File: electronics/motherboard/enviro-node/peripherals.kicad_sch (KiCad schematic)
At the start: 9 parts, among them J5 ST1W008S4AR1500, J6 2604-3105, Q3 BSS214NW, U3 TCA9534

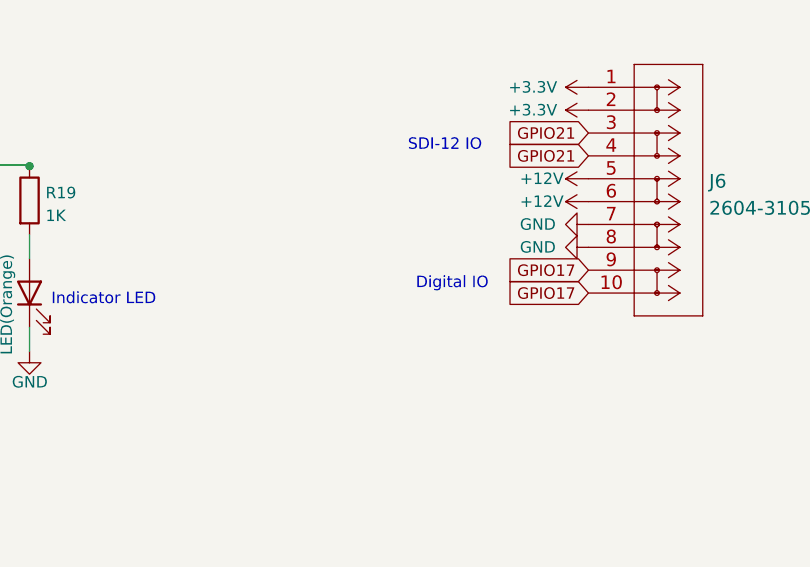
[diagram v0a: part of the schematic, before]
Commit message: updated electronics for production
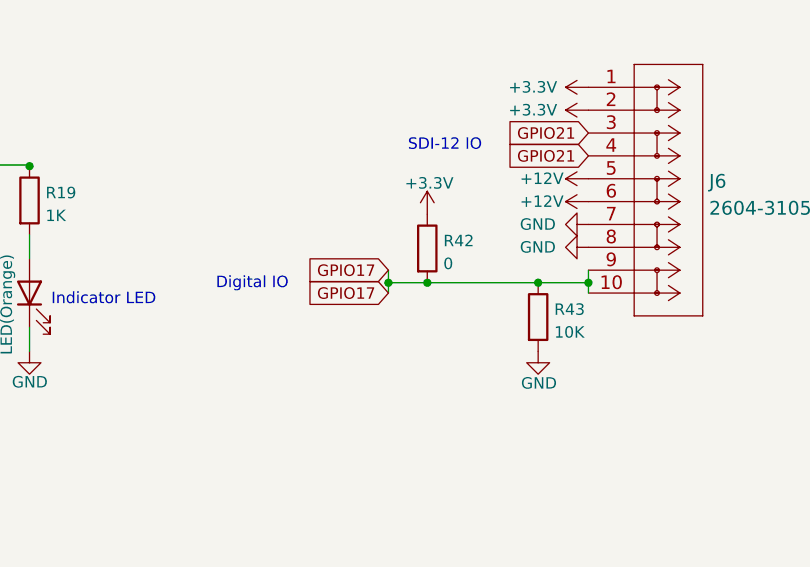
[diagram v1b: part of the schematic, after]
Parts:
- added R42: 0, Resistor_SMD:R_0805_2012Metric, symbol Device:R
- added R43: 10K, Resistor_SMD:R_0805_2012Metric, symbol Device:R
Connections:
- net +3.3V: now also R42.1
- net GND: now also R43.2
- net GPIO17: now also R42.2, R43.1
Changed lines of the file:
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@@
   (junction (at 119.507 115.697) (diameter 0) (color 0 0 0 0)
   )
+  (junction (at 230.632 116.078) (diameter 0) (color 0 0 0 0)
+  )
+  (junction (at 213.995 116.078) (diameter 0) (color 0 0 0 0)
+  )
   (junction (at 119.507 118.237) (diameter 0) (color 0 0 0 0)
   )
   (junction (at 174.117 103.124) (diameter 0) (color 0 0 0 0)
+  )
+  (junction (at 218.313 116.078) (diameter 0) (color 0 0 0 0)
+  )
+  (junction (at 236.22 116.078) (diameter 0) (color 0 0 0 0)
   )
   (no_connect (at 119.507 105.537))
@@
     (stroke (width 0) (type default) (color 0 0 0 0))
   )
+  (wire (pts (xy 236.22 114.681) (xy 236.22 116.078))
+    (stroke (width 0) (type default) (color 0 0 0 0))
+  )
+  (wire (pts (xy 213.995 116.078) (xy 213.995 117.221))
+    (stroke (width 0) (type default) (color 0 0 0 0))
+  )
   (wire (pts (xy 58.928 104.902) (xy 46.101 104.902))
     (stroke (width 0) (type default) (color 0 0 0 0))
   )
+  (wire (pts (xy 213.995 116.078) (xy 218.313 116.078))
+    (stroke (width 0) (type default) (color 0 0 0 0))
+  )
   (wire (pts (xy 174.117 102.997) (xy 174.117 103.124))
     (stroke (width 0) (type default) (color 0 0 0 0))
@@
     (stroke (width 0) (type default) (color 0 0 0 0))
   )
+  (wire (pts (xy 236.22 116.078) (xy 236.22 117.221))
+    (stroke (width 0) (type default) (color 0 0 0 0))
+  )
+  (wire (pts (xy 230.632 116.078) (xy 236.22 116.078))
+    (stroke (width 0) (type default) (color 0 0 0 0))
+  )
   (wire (pts (xy 58.928 125.222) (xy 58.928 104.902))
     (stroke (width 0) (type default) (color 0 0 0 0))
   )
+  (wire (pts (xy 218.313 116.078) (xy 230.632 116.078))
+    (stroke (width 0) (type default) (color 0 0 0 0))
+  )
   (wire (pts (xy 139.827 102.997) (xy 174.117 102.997))
     (stroke (width 0) (type default) (color 0 0 0 0))
   )
+  (wire (pts (xy 213.995 114.681) (xy 213.995 116.078))
+    (stroke (width 0) (type default) (color 0 0 0 0))
+  )
   (wire (pts (xy 119.507 115.697) (xy 119.507 118.237))
     (stroke (width 0) (type default) (color 0 0 0 0))
@@
     (stroke (width 0) (type default) (color 0 0 0 0))
   )
-  (text "Digital IO" (at 217.043 116.967 0)
+  (text "Digital IO" (at 194.818 116.967 0)
     (effects (font (size 1.27 1.27)) (justify left bottom))
   )
@@
     )
   )
-  (global_label "GPIO17" (shape input) (at 236.22 114.681 180) (fields_autoplaced)
-    (effects (font (size 1.27 1.27)) (justify right))
-    (property "Intersheet References" "${INTERSHEET_REFS}" (id 0) (at 226.9126 114.6016 0)
+  (global_label "GPIO17" (shape input) (at 213.995 114.681 180) (fields_autoplaced)
+    (effects (font (size 1.27 1.27)) (justify right))
+    (property "Intersheet References" "${INTERSHEET_REFS}" (id 0) (at 204.6876 114.6016 0)
       (effects (font (size 1.27 1.27)) (justify right) hide)
     )
@@
     )
   )
-  (global_label "GPIO17" (shape input) (at 236.22 117.221 180) (fields_autoplaced)
-    (effects (font (size 1.27 1.27)) (justify right))
-    (property "Intersheet References" "${INTERSHEET_REFS}" (id 0) (at 226.9126 117.1416 0)
+  (global_label "GPIO17" (shape input) (at 213.995 117.221 180) (fields_autoplaced)
+    (effects (font (size 1.27 1.27)) (justify right))
+    (property "Intersheet References" "${INTERSHEET_REFS}" (id 0) (at 204.6876 117.1416 0)
       (effects (font (size 1.27 1.27)) (justify right) hide)
     )
@@
     (pin "2")
     (pin "3")
+  )
+  (symbol (lib_id "Device:R") (at 218.313 112.268 0) (unit 1)
+    (in_bom yes) (on_board yes)
+    (property "Reference" "R42" (id 0) (at 220.091 111.4333 0)
+      (effects (font (size 1.27 1.27)) (justify left))
+    )
+    (property "Value" "0" (id 1) (at 220.091 113.9702 0)
+      (effects (font (size 1.27 1.27)) (justify left))
+    )
+    (property "Footprint" "Resistor_SMD:R_0805_2012Metric" (id 2) (at 216.535 112.268 90)
+      (effects (font (size 1.27 1.27)) hide)
+    )
+    (property "Datasheet" "~" (id 3) (at 218.313 112.268 0)
+      (effects (font (size 1.27 1.27)) hide)
+    )
+    (property "Populate" "False" (id 4) (at 218.313 112.268 0)
+      (effects (font (size 1.27 1.27)) hide)
+    )
+    (pin "1")
+    (pin "2")
   )
   (symbol (lib_id "power:+12V") (at 236.22 107.061 90) (unit 1)
@@
     (pin "1")
   )
+  (symbol (lib_id "power:+3.3V") (at 218.313 108.458 0) (unit 1)
+    (in_bom yes) (on_board yes)
+    (property "Reference" "#PWR0117" (id 0) (at 218.313 112.268 0)
+      (effects (font (size 1.27 1.27)) hide)
+    )
+    (property "Value" "+3.3V" (id 1) (at 221.234 105.029 0)
+      (effects (font (size 1.27 1.27)) (justify right))
+    )
+    (property "Footprint" "" (id 2) (at 218.313 108.458 0)
+      (effects (font (size 1.27 1.27)) hide)
+    )
+    (property "Datasheet" "" (id 3) (at 218.313 108.458 0)
+      (effects (font (size 1.27 1.27)) hide)
+    )
+    (pin "1")
+  )
+  (symbol (lib_id "power:GND") (at 230.632 123.698 0) (unit 1)
+    (in_bom yes) (on_board yes)
+    (property "Reference" "#PWR0116" (id 0) (at 230.632 130.048 0)
+      (effects (font (size 1.27 1.27)) hide)
+    )
+    (property "Value" "GND" (id 1) (at 228.727 127.254 0)
+      (effects (font (size 1.27 1.27)) (justify left))
+    )
+    (property "Footprint" "" (id 2) (at 230.632 123.698 0)
+      (effects (font (size 1.27 1.27)) hide)
+    )
+    (property "Datasheet" "" (id 3) (at 230.632 123.698 0)
+      (effects (font (size 1.27 1.27)) hide)
+    )
+    (pin "1")
+  )
   (symbol (lib_id "power:GND") (at 236.22 112.141 270) (unit 1)
     (in_bom yes) (on_board yes)
@@
       (effects (font (size 1.27 1.27)) hide)
     )
+    (pin "1")
+    (pin "2")
+  )
+  (symbol (lib_id "Device:R") (at 230.632 119.888 0) (unit 1)
+    (in_bom yes) (on_board yes)
+    (property "Reference" "R43" (id 0) (at 232.41 119.0533 0)
+      (effects (font (size 1.27 1.27)) (justify left))
+    )
+    (property "Value" "10K" (id 1) (at 232.41 121.5902 0)
+      (effects (font (size 1.27 1.27)) (justify left))
+    )
+    (property "Footprint" "Resistor_SMD:R_0805_2012Metric" (id 2) (at 228.854 119.888 90)
+      (effects (font (size 1.27 1.27)) hide)
+    )
+    (property "Datasheet" "~" (id 3) (at 230.632 119.888 0)
+      (effects (font (size 1.27 1.27)) hide)
+    )
